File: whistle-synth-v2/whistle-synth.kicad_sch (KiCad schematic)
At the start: 21 parts

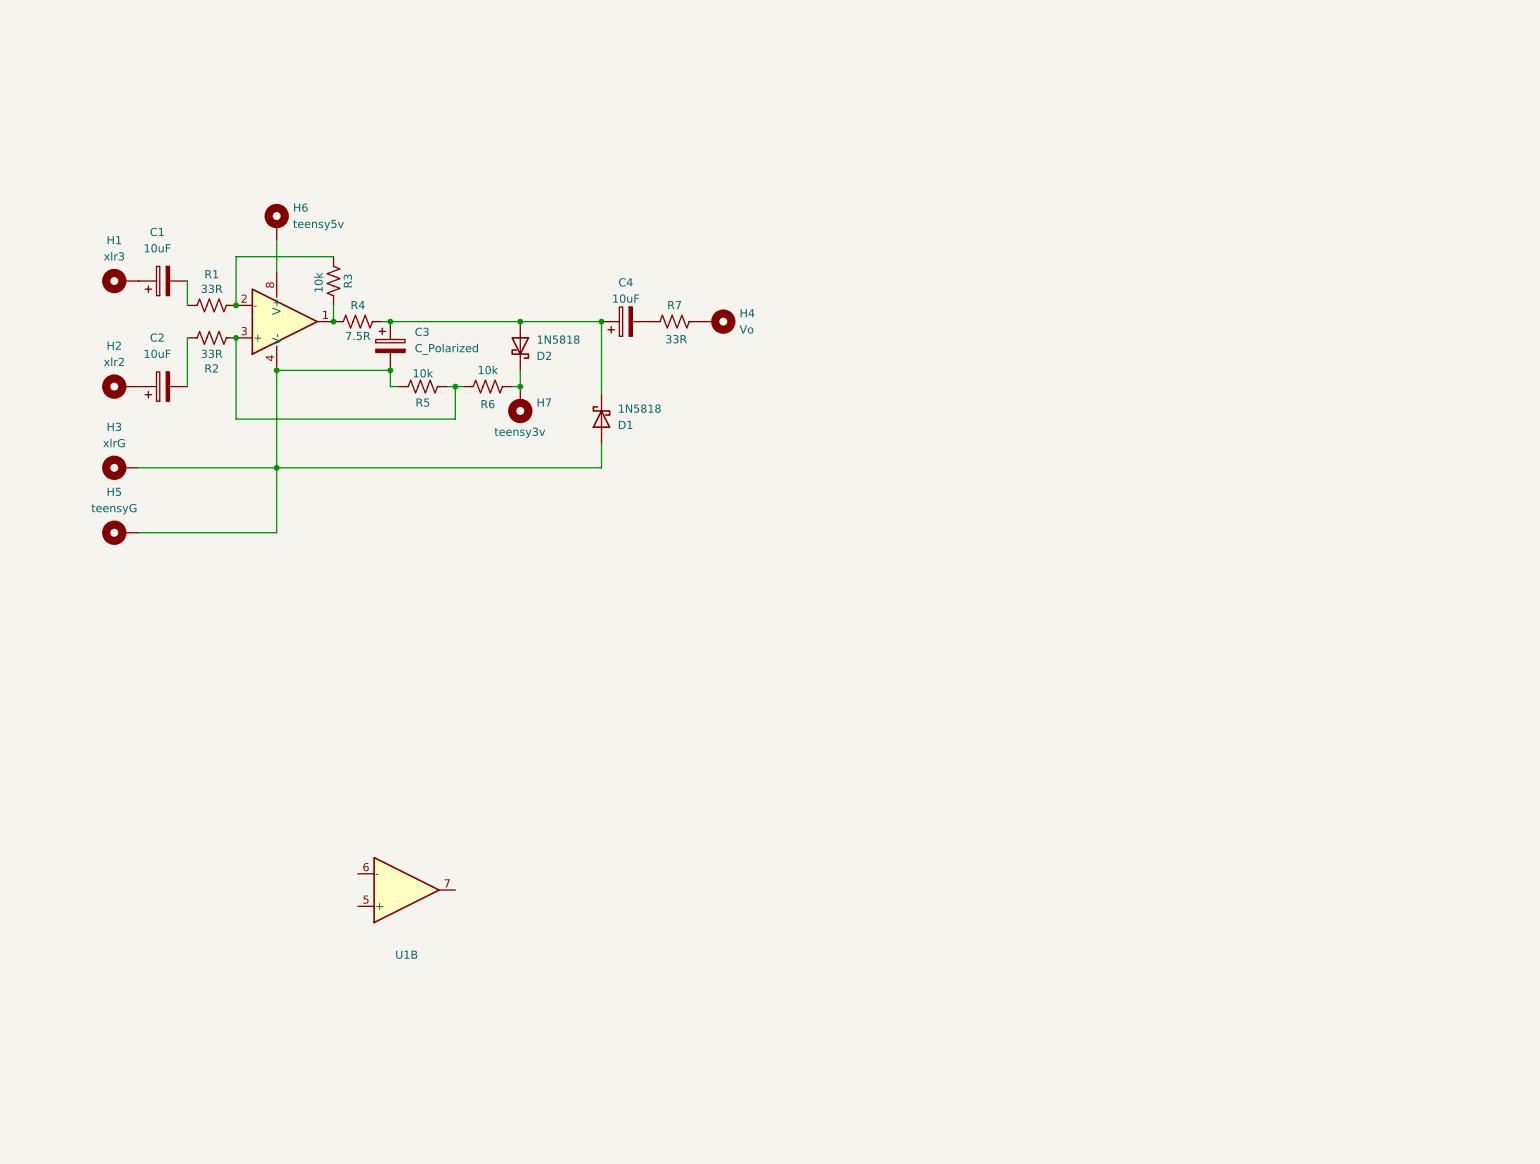
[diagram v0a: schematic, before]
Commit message: check in
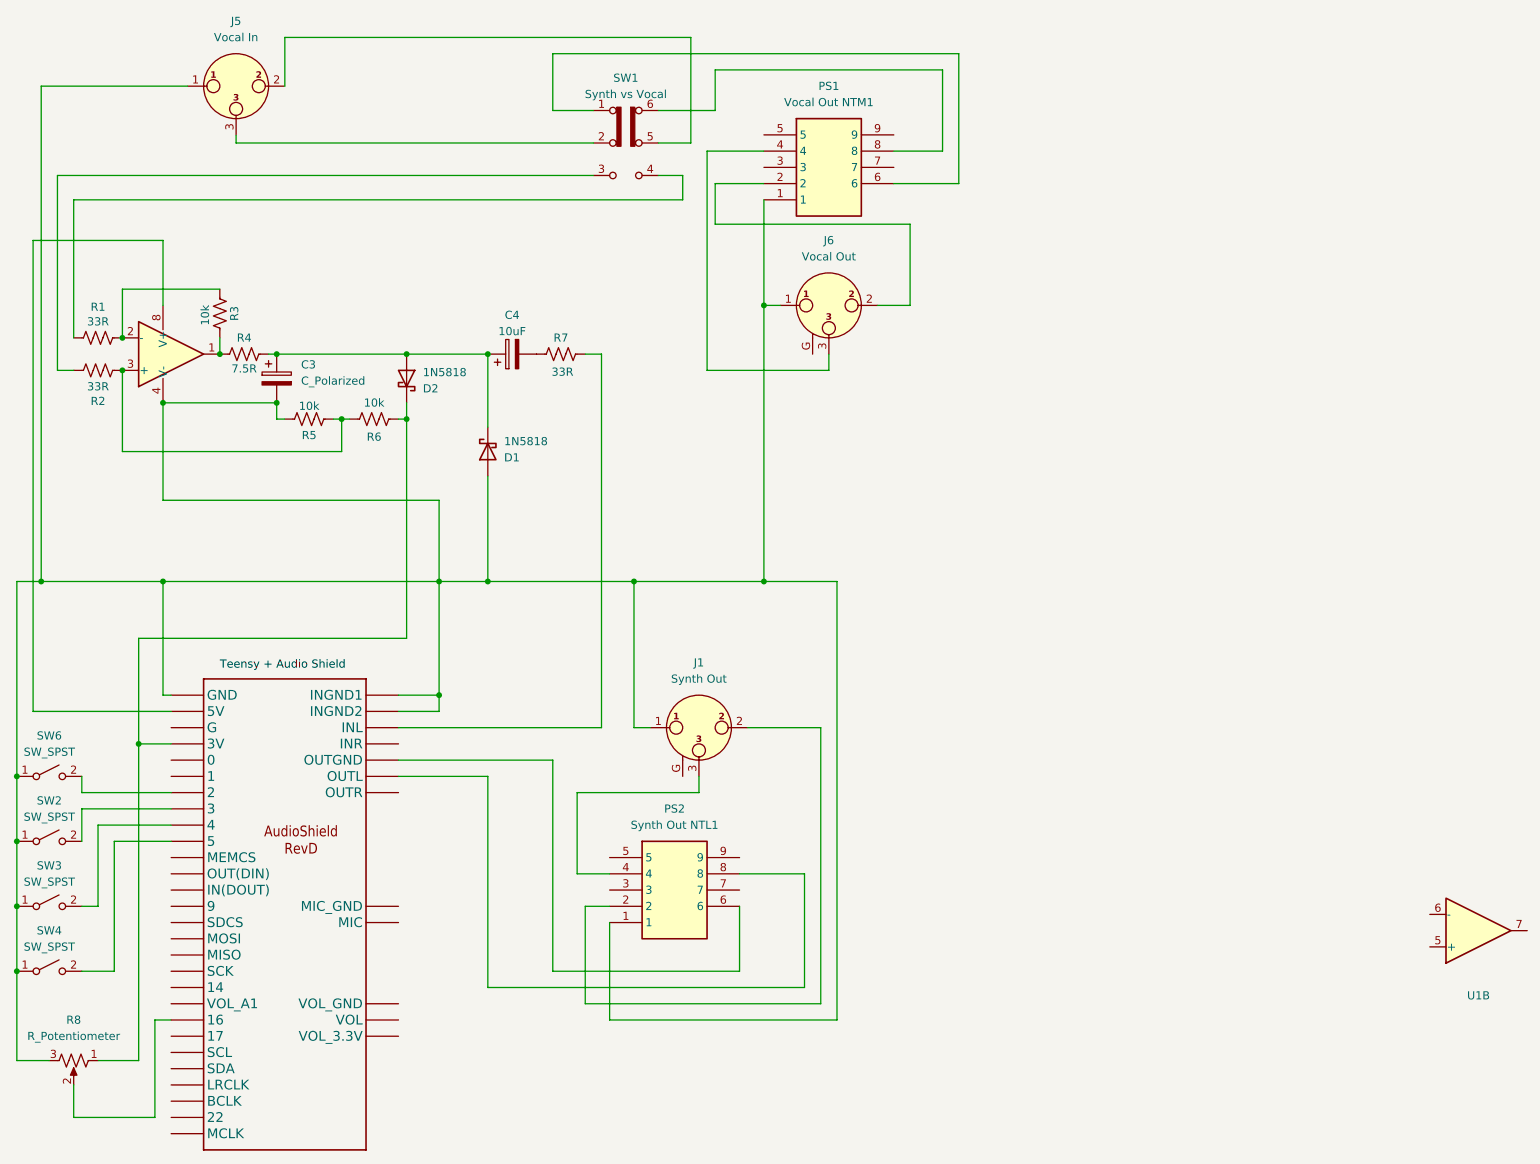
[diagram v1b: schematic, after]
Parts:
- removed C1, C2: 10uF, Capacitor_THT:CP_Radial_D4.0mm_P2.00mm, symbol Device:C_Polarized
- removed H1: xlr3, MountingHole:MountingHole_2.2mm_M2_DIN965_Pad_TopBottom, symbol Mechanical:MountingHole_Pad
- removed H2: xlr2, MountingHole:MountingHole_2.2mm_M2_DIN965_Pad_TopBottom, symbol Mechanical:MountingHole_Pad
- removed H3: xlrG, MountingHole:MountingHole_2.2mm_M2_DIN965_Pad_TopBottom, symbol Mechanical:MountingHole_Pad
- removed H4: Vo, MountingHole:MountingHole_2.2mm_M2_DIN965_Pad_TopBottom, symbol Mechanical:MountingHole_Pad
- removed H5: teensyG, MountingHole:MountingHole_2.2mm_M2_DIN965_Pad_TopBottom, symbol Mechanical:MountingHole_Pad
- removed H6: teensy5v, MountingHole:MountingHole_2.2mm_M2_DIN965_Pad_TopBottom, symbol Mechanical:MountingHole_Pad
- removed H7: teensy3v, MountingHole:MountingHole_2.2mm_M2_DIN965_Pad_TopBottom, symbol Mechanical:MountingHole_Pad
- added 1: ~, symbol Teensy_Audioshield:AUDIOSHIELD-REVD
- added J1: Synth Out, Connector_Audio:Jack_XLR_Neutrik_NC3MAH_Horizontal, symbol Connector_Audio:NC3MAH
- added J5: Vocal In, Connector_Audio:Jack_XLR_Neutrik_NC3FAAH_Horizontal, symbol Connector_Audio:NC3FAAH
- added J6: Vocal Out, Connector_Audio:Jack_XLR_Neutrik_NC3MAH_Horizontal, symbol Connector_Audio:NC3MAH
- added PS1: Vocal Out NTM1, Library:NTL1, symbol NTL1:NTL1
- added PS2: Synth Out NTL1, Library:NTL1, symbol NTL1:NTL1
- added R8: R_Potentiometer, PCM_SparkFun-Resistor:Bourns-PDB18, symbol PCM_SparkFun-Resistor:R_Potentiometer
- added SW1: Synth vs Vocal, Button_Switch_THT:SW_Push_2P2T_Toggle_CK_PVA2xxH1xxxxxxV2, symbol Switch:SW_Slide_DPDT
- added SW2, SW3, SW4, SW6: SW_SPST, Button_Switch_THT:SW_DIP_SPSTx01_Slide_9.78x4.72mm_W7.62mm_P2.54mm, symbol Switch:SW_SPST
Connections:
- net at C3.2, D1.2 (A), R5.2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: now also 1.GND, 1.INGND1, 1.INGND2, J1.1, J5.1, J6.1, PS1.1, PS2.1, R8.3, SW2.1 (A), SW3.1 (A), SW4.1 (A), SW6.1 (A)
- net at R1.2: now also SW1.4 (A)
- net at U1.8 (V+): now also 1.5V
- net at D2.1 (K), R6.1: now also 1.3V, R8.1
- net at R7.1: now also 1.INL
- net at R2.2: now also SW1.3 (C)
- new net: 1.2, SW6.2 (B)
- new net: 1.3, SW2.2 (B)
- new net: 1.16, R8.2
- new net: J6.2, PS1.2
- new net: J6.3, PS1.4
- new net: PS1.6, SW1.1 (A)
- new net: PS1.8, SW1.6 (C)
- new net: 1.4, SW3.2 (B)
- new net: 1.5, SW4.2 (B)
- new net: 1.OUTGND, PS2.6
- new net: 1.OUTL, PS2.8
- new net: J1.2, PS2.2
- new net: J1.3, PS2.4
- new net: J5.2, SW1.5 (B)
- new net: J5.3, SW1.2 (B)
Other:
- moved on the sheet: C3, C4, D1, D2, R1, R2, R3, R4, R5, R6, R7, U1B
